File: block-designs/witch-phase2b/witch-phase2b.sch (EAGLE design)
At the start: 69 parts, among them IC1 74HC160N, IC10 74LS73N, IC11 74LS08N, IC12 74LS32N, IC2 4511N, IC3 74HC160N, IC4 4511N, IC5 74HC160N, IC6 4511N, IC7 74HC160N, IC8 4511N, IC9 74LS73N

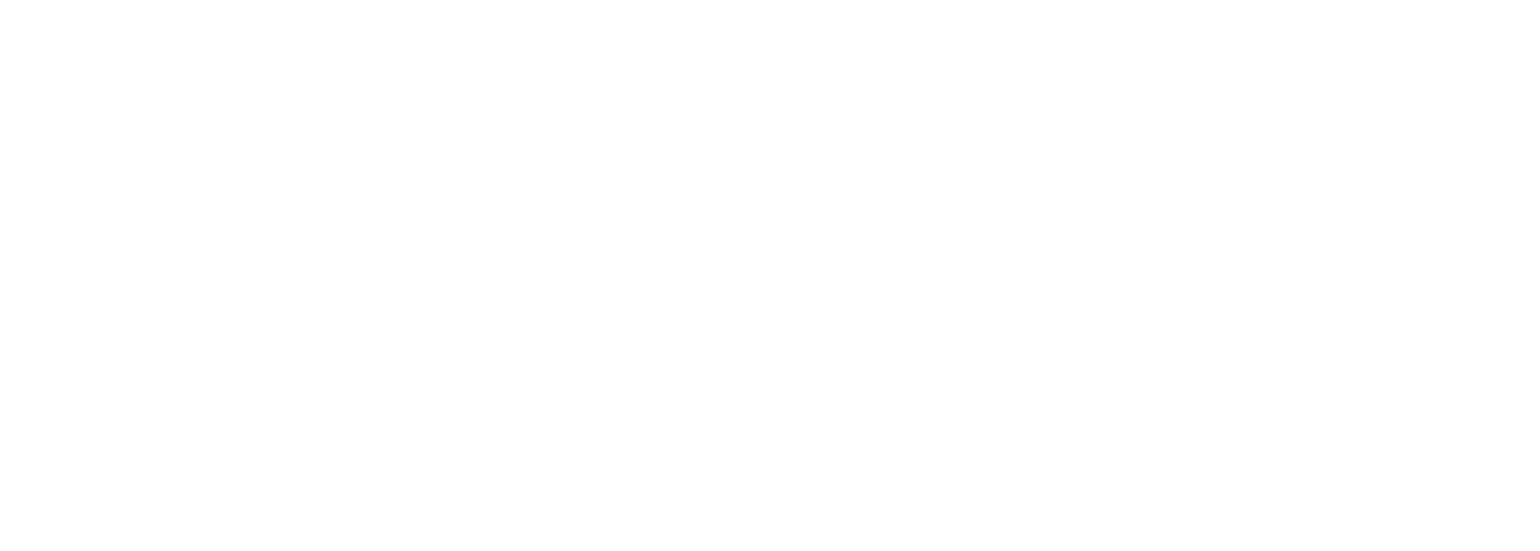
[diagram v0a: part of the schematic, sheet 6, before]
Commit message: updated board layouts
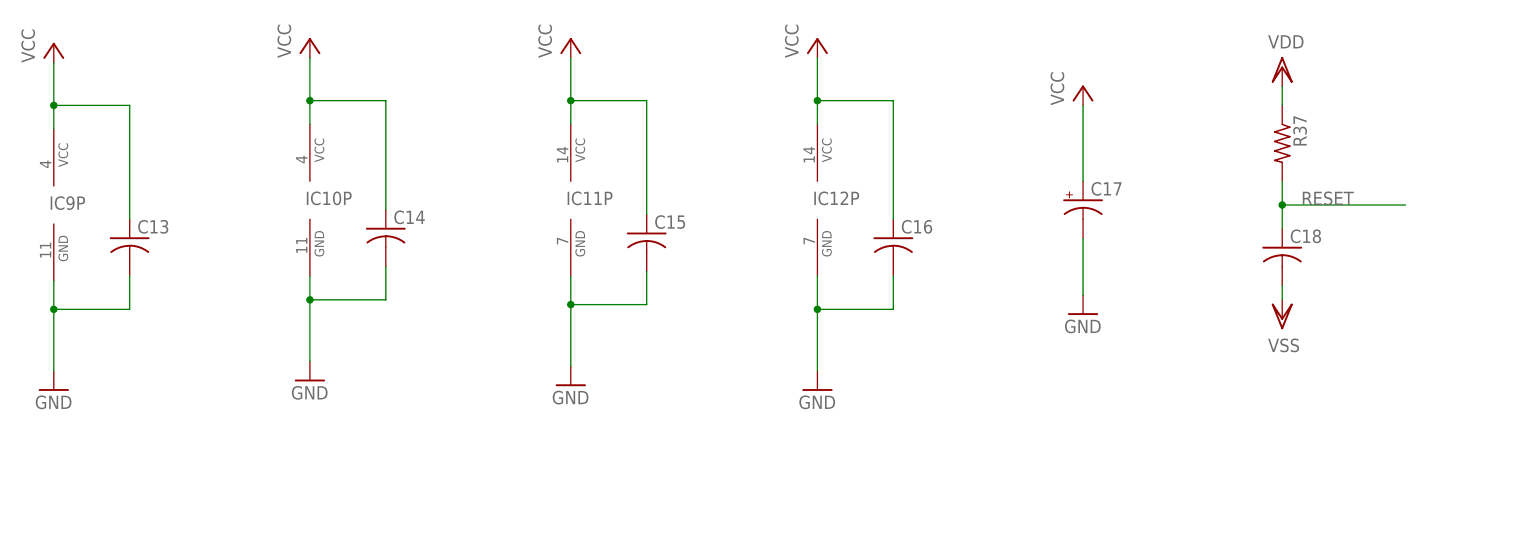
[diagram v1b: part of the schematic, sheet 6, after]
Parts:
- added C13, C14, C15, C16: (no value), resistor:C-US025-025X050
- added C17: (no value), resistor:CPOL-USE2-5
- added C18: (no value), resistor:C-US025-040X050
- added R37: (no value), resistor:R-US_0204/5
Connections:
- new net VDD: R37.1
- new net VSS: C18.2
- net GND: now also C13.2, C14.2, C15.2, C16.2, C17.-, IC10P.GND, IC11P.GND, IC12P.GND, IC9P.GND
- net RESET: now also C18.1, R37.2
- net VCC: now also C13.1, C14.1, C15.1, C16.1, C17.+, IC10P.VCC, IC11P.VCC, IC12P.VCC, IC9P.VCC
